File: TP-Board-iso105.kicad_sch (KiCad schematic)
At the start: 425 parts, among them SW1 SW_Push, SW10 SW_Push, SW100 SW_Push, SW101 SW_Push, SW102 SW_Push, SW103 SW_Push, SW104 SW_Push, SW105 SW_Push, SW11 SW_Push, SW12 SW_Push, SW13 SW_Push, SW14 SW_Push, SW15 SW_Push, SW16 SW_Push, SW17 SW_Push, SW18 SW_Push, SW19 SW_Push, SW2 SW_Push, SW20 SW_Push, SW21 SW_Push, SW22 SW_Push, SW23 SW_Push, SW24 SW_Push, SW25 SW_Push, SW26 SW_Push, SW27 SW_Push, SW28 SW_Push, SW29 SW_Push, SW3 SW_Push, SW30 SW_Push, SW31 SW_Push, SW32 SW_Push, SW33 SW_Push, SW34 SW_Push, SW35 SW_Push, SW36 SW_Push, SW37 SW_Push, SW38 SW_Push, SW39 SW_Push, SW4 SW_Push, SW40 SW_Push, SW41 SW_Push, SW42 SW_Push, SW43 SW_Push, SW44 SW_Push, SW45 SW_Push, SW46 SW_Push, SW47 SW_Push, SW48 SW_Push, SW49 SW_Push, SW5 SW_Push, SW50 SW_Push, SW51 SW_Push, SW52 SW_Push, SW53 SW_Push, SW54 SW_Push, SW55 SW_Push, SW56 SW_Push, SW57 SW_Push, SW58 SW_Push, SW59 SW_Push, SW6 SW_Push, SW60 SW_Push, SW61 SW_Push, SW62 SW_Push, SW63 SW_Push, SW64 SW_Push, SW65 SW_Push, SW66 SW_Push, SW67 SW_Push, SW68 SW_Push, SW69 SW_Push, SW7 SW_Push, SW70 SW_Push, SW71 SW_Push, SW72 SW_Push, SW73 SW_Push, SW74 SW_Push, SW75 SW_Push, SW76 SW_Push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

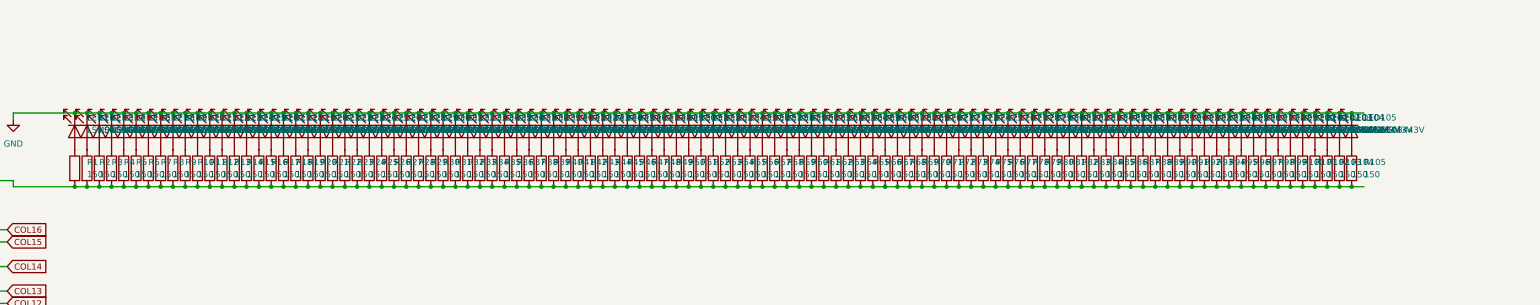
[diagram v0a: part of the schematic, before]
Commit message: 💀
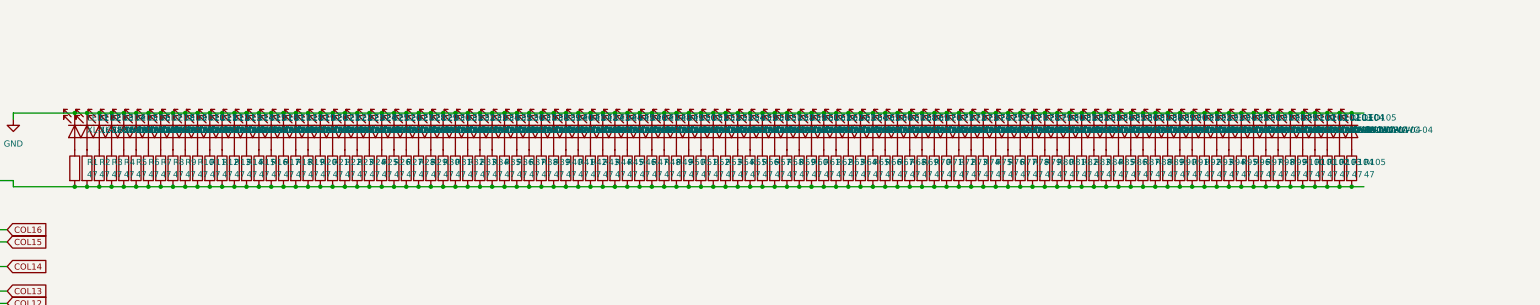
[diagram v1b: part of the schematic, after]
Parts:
- H1, H2, H3, H4, SW1, SW10, SW100, SW101, SW102, SW103, SW104, SW105, SW11, SW12, SW13, SW14, SW15, SW16, SW17, SW18, SW19, SW2, SW20, SW21, SW22, SW23, SW24, SW25, SW26, SW27, SW28, SW29, SW3, SW30, SW31, SW32, SW33, SW34, SW35, SW36, SW37, SW38, SW39, SW4, SW40, SW41, SW42, SW43, SW44, SW45, SW46, SW47, SW48, SW49, SW5, SW50, SW51, SW52, SW53, SW54, SW55, SW56, SW57, SW58, SW59, SW6, SW60, SW61, SW62, SW63, SW64, SW65, SW66, SW67, SW68, SW69, SW7, SW70, SW71, SW72, SW73, SW74, SW75, SW76, SW77, SW78, SW79, SW8, SW80, SW81, SW82, SW83, SW84, SW85, SW86, SW87, SW88, SW89, SW9, SW90, SW91, SW92, SW93, SW94, SW95, SW96, SW97, SW98, SW99, U1: now left out of the parts list
- LED1, LED10, LED100, LED101, LED102, LED103, LED104, LED105, LED11, LED12, LED13, LED14, LED15, LED16, LED17, LED18, LED19, LED2, LED20, LED21, LED22, LED23, LED24, LED25, LED26, LED27, LED28, LED29, LED3, LED30, LED31, LED32, LED33, LED34, LED35, LED36, LED37, LED38, LED39, LED4, LED40, LED41, LED42, LED43, LED44, LED45, LED46, LED47, LED48, LED49, LED5, LED50, LED51, LED52, LED53, LED54, LED55, LED56, LED57, LED58, LED59, LED6, LED60, LED61, LED62, LED63, LED64, LED65, LED66, LED67, LED68, LED69, LED7, LED70, LED71, LED72, LED73, LED74, LED75, LED76, LED77, LED78, LED79, LED8, LED80, LED81, LED82, LED83, LED84, LED85, LED86, LED87, LED88, LED89, LED9, LED90, LED91, LED92, LED93, LED94, LED95, LED96, LED97, LED98, LED99: value LSM0603443V -> XL-1608UWC-04
- R1, R10, R100, R101, R102, R103, R104, R105, R11, R12, R13, R14, R15, R16, R17, R18, R19, R2, R20, R21, R22, R23, R24, R25, R26, R27, R28, R29, R3, R30, R31, R32, R33, R34, R35, R36, R37, R38, R39, R4, R40, R41, R42, R43, R44, R45, R46, R47, R48, R49, R5, R50, R51, R52, R53, R54, R55, R56, R57, R58, R59, R6, R60, R61, R62, R63, R64, R65, R66, R67, R68, R69, R7, R70, R71, R72, R73, R74, R75, R76, R77, R78, R79, R8, R80, R81, R82, R83, R84, R85, R86, R87, R88, R89, R9, R90, R91, R92, R93, R94, R95, R96, R97, R98, R99: value 150 -> 47; footprint Resistor_SMD:R_0201_0603Metric_Pad0.64x0.40mm_HandSolder -> Resistor_SMD:R_0603_1608Metric
